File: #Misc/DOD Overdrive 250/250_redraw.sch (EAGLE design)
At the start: 21 parts, among them IC1 LM741, J1 IN, J2 OUT

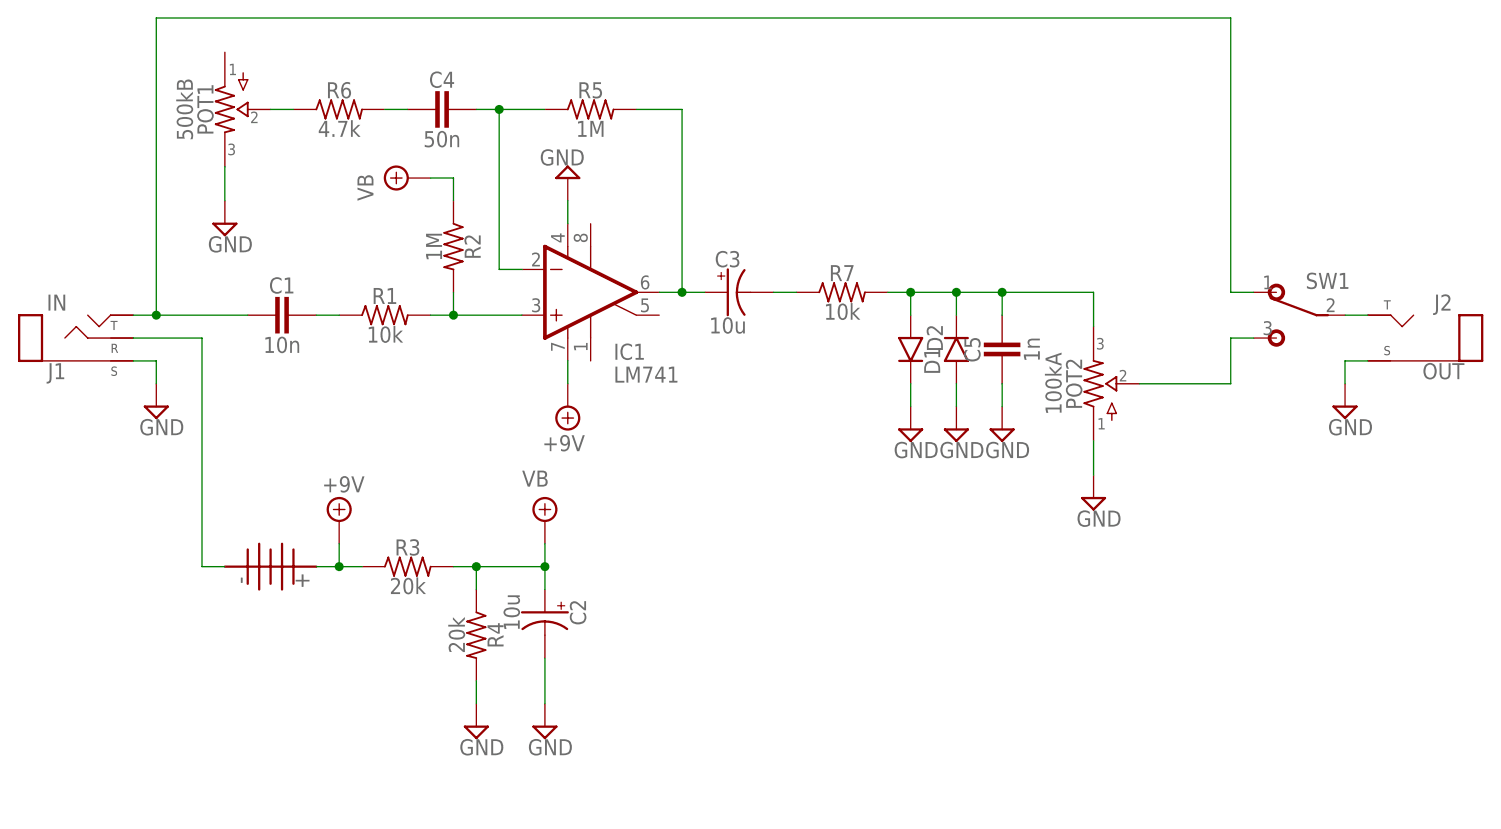
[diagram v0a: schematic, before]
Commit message: 20180125
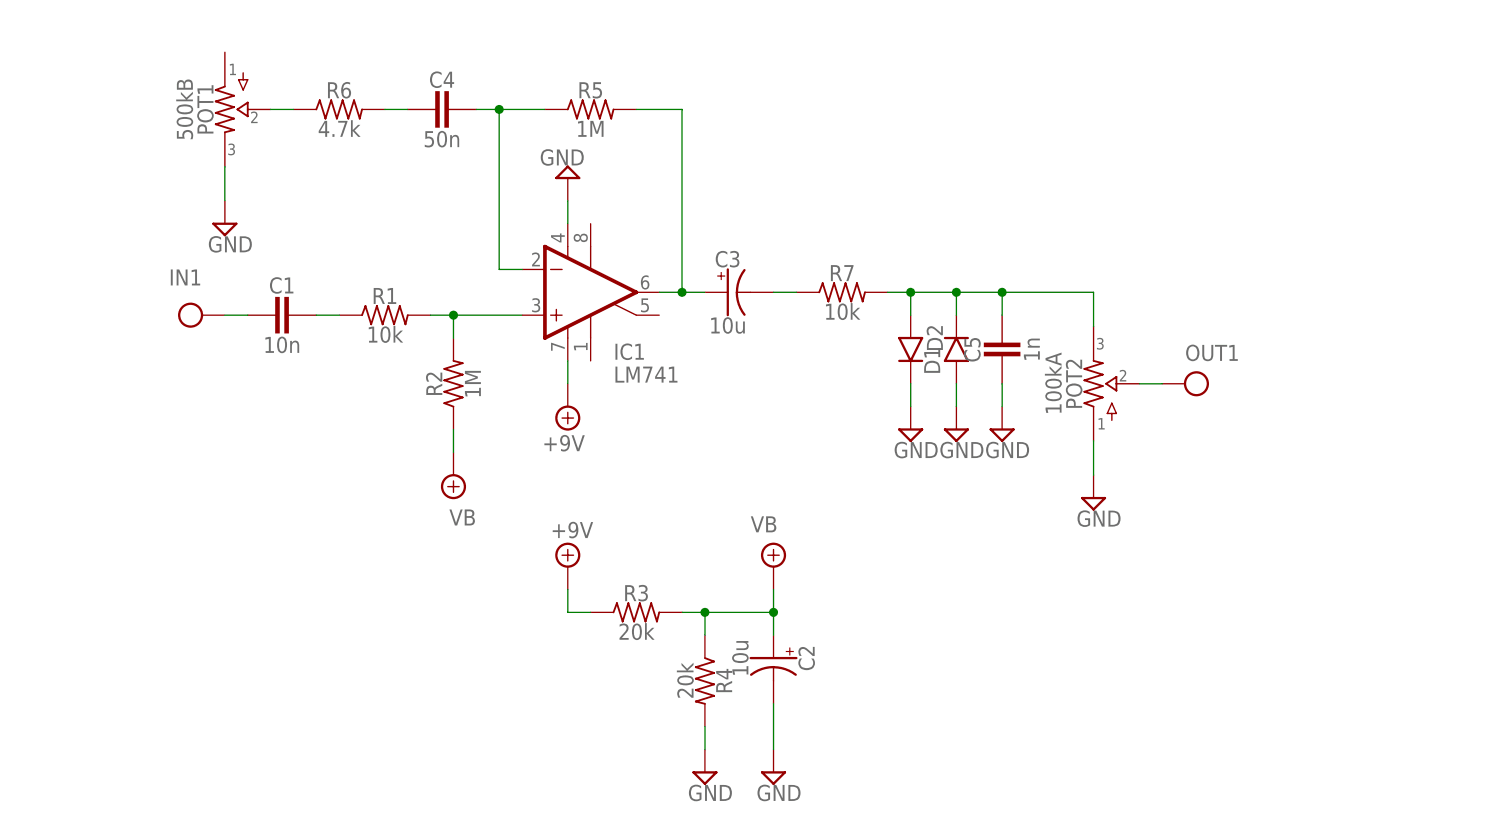
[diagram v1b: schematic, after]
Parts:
- removed 1: 9V, pedals-jacks:BATTERY
- removed J1: IN, pedals-jacks:STEREO
- removed J2: OUT, pedals-jacks:MONO_JACK
- removed SW1: (no value), pedals-switches:SPDT
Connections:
- removed net N$1: 1.P$2, J1.R
- removed net N$14: POT2.2, SW1.S
- removed net N$3: J1.T, SW1.O
- removed net N$6: J2.TIP, SW1.P
- new net IN: C1.2
- new net OUT: POT2.2
- net +9V: no longer 1.P$1
- net GND: no longer J1.S, J2.SLEEVE
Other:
- moved on the sheet: C2, R2, R3, R4
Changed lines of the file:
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@@
 <?xml version="1.0" encoding="utf-8"?>
 <!DOCTYPE eagle SYSTEM "eagle.dtd">
-<eagle version="8.2.0">
+<eagle version="8.5.1">
 <drawing>
 <settings>
 <setting alwaysvectorfont="no"/>
+<setting keepoldvectorfont="yes"/>
 <setting verticaltext="up"/>
 </settings>
-<grid distance="0.1" unitdist="inch" unit="inch" style="lines" multiple="1" display="yes" altdistance="0.01" altunitdist="inch" altunit="inch"/>
+<grid distance="0.1" unitdist="inch" unit="inch" style="lines" multiple="1" display="no" altdistance="0.01" altunitdist="inch" altunit="inch"/>
 <layers>
 <layer number="1" name="Top" color="4" fill="1" visible="no" active="no"/>
@@
 <layer number="59" name="tCarbon" color="7" fill="1" visible="no" active="no"/>
 <layer number="60" name="bCarbon" color="7" fill="1" visible="no" active="no"/>
+<layer number="88" name="SimResults" color="9" fill="1" visible="yes" active="yes"/>
+<layer number="89" name="SimProbes" color="9" fill="1" visible="yes" active="yes"/>
 <layer number="90" name="Modules" color="5" fill="1" visible="yes" active="yes"/>
 <layer number="91" name="Nets" color="2" fill="1" visible="yes" active="yes"/>
@@
 </classes>
 <parts>
-<part name="J1" library="pedals-jacks" deviceset="STEREO" device="" value="IN"/>
-<part name="GND1" library="gm-supply" deviceset="GND" device=""/>
-<part name="1" library="pedals-jacks" deviceset="BATTERY" device="" value="9V"/>
-<part name="J2" library="pedals-jacks" deviceset="MONO" device="_JACK" value="OUT"/>
 <part name="C1" library="pedals-capacitors-film" deviceset="CER/FILM" device="BOX.1" value="10n"/>
-<part name="SW1" library="pedals-switches" deviceset="SPDT" device=""/>
 <part name="R1" library="pedals-resistors" deviceset="R_" device=".3B" value="10k"/>
 <part name="R2" library="pedals-resistors" deviceset="R_" device=".3B" value="1M"/>
@@
 <part name="VB2" library="gm-supply" deviceset="VB" device=""/>
 <part name="V2" library="gm-supply" deviceset="+9V" device=""/>
-<part name="GND10" library="gm-supply" deviceset="GND" device=""/>
+<part name="IN1" library="pedals-supply" deviceset="IN" device=""/>
+<part name="OUT1" library="pedals-supply" deviceset="OUT" device=""/>
 </parts>
 <sheets>
@@
 </plain>
 <instances>
-<instance part="J1" gate="G$1" x="2.54" y="66.04" rot="MR180"/>
-<instance part="GND1" gate="GND" x="17.78" y="55.88"/>
-<instance part="1" gate="G$1" x="30.48" y="38.1" rot="R270"/>
-<instance part="J2" gate="G$1" x="157.48" y="63.5" rot="MR0"/>
 <instance part="C1" gate="G$1" x="31.75" y="66.04"/>
-<instance part="SW1" gate="1" x="144.78" y="68.58" rot="MR270"/>
 <instance part="R1" gate="G$1" x="43.18" y="66.04"/>
-<instance part="R2" gate="G$1" x="50.8" y="73.66" rot="R270"/>
-<instance part="R3" gate="G$1" x="45.72" y="38.1"/>
-<instance part="R4" gate="G$1" x="53.34" y="30.48" rot="R270"/>
-<instance part="C2" gate="1" x="60.96" y="33.02" rot="R270"/>
-<instance part="GND2" gate="GND" x="53.34" y="20.32"/>
+<instance part="R2" gate="G$1" x="50.8" y="58.42" rot="R90"/>
+<instance part="R3" gate="G$1" x="71.12" y="33.02"/>
+<instance part="R4" gate="G$1" x="78.74" y="25.4" rot="R270"/>
+<instance part="C2" gate="1" x="86.36" y="27.94" rot="R270"/>
+<instance part="GND2" gate="GND" x="78.74" y="15.24"/>
 <instance part="IC1" gate="A" x="66.04" y="68.58" rot="MR180"/>
 <instance part="GND3" gate="GND" x="63.5" y="81.28" rot="R180"/>
@@
 <instance part="GND7" gate="GND" x="111.76" y="53.34"/>
 <instance part="GND8" gate="GND" x="121.92" y="45.72"/>
-<instance part="GND9" gate="GND" x="60.96" y="20.32"/>
-<instance part="V1" gate="+9V" x="38.1" y="43.18"/>
-<instance part="VB1" gate="G$1" x="60.96" y="43.18"/>
-<instance part="VB2" gate="G$1" x="45.72" y="81.28" rot="R90"/>
+<instance part="GND9" gate="GND" x="86.36" y="15.24"/>
+<instance part="V1" gate="+9V" x="63.5" y="38.1"/>
+<instance part="VB1" gate="G$1" x="86.36" y="38.1"/>
+<instance part="VB2" gate="G$1" x="50.8" y="48.26" rot="R180"/>
 <instance part="V2" gate="+9V" x="63.5" y="55.88" rot="R180"/>
-<instance part="GND10" gate="GND" x="149.86" y="55.88"/>
+<instance part="IN1" gate="G$1" x="22.86" y="66.04"/>
+<instance part="OUT1" gate="G$1" x="132.08" y="58.42"/>
 </instances>
 <busses>
 </busses>
 <nets>
-<net name="N$1" class="0">
-<segment>
-<pinref part="J1" gate="G$1" pin="R"/>
-<wire x1="15.24" y1="63.5" x2="22.86" y2="63.5" width="0.1524" layer="91"/>
-<wire x1="22.86" y1="63.5" x2="22.86" y2="38.1" width="0.1524" layer="91"/>
-<pinref part="1" gate="G$1" pin="P$2"/>
-<wire x1="22.86" y1="38.1" x2="25.4" y2="38.1" width="0.1524" layer="91"/>
-</segment>
-</net>
-<net name="N$3" class="0">
-<segment>
-<pinref part="J1" gate="G$1" pin="T"/>
-<wire x1="15.24" y1="66.04" x2="17.78" y2="66.04" width="0.1524" layer="91"/>
-<pinref part="SW1" gate="1" pin="O"/>
-<wire x1="17.78" y1="66.04" x2="27.94" y2="66.04" width="0.1524" layer="91"/>
-<wire x1="139.7" y1="68.58" x2="137.16" y2="68.58" width="0.1524" layer="91"/>
-<wire x1="137.16" y1="68.58" x2="137.16" y2="99.06" width="0.1524" layer="91"/>
-<wire x1="137.16" y1="99.06" x2="17.78" y2="99.06" width="0.1524" layer="91"/>
-<wire x1="17.78" y1="99.06" x2="17.78" y2="66.04" width="0.1524" layer="91"/>
-<junction x="17.78" y="66.04"/>
-</segment>
-</net>
 <net name="GND" class="0">
-<segment>
-<pinref part="J1" gate="G$1" pin="S"/>
-<pinref part="GND1" gate="GND" pin="GND"/>
-<wire x1="15.24" y1="60.96" x2="17.78" y2="60.96" width="0.1524" layer="91"/>
-<wire x1="17.78" y1="60.96" x2="17.78" y2="58.42" width="0.1524" layer="91"/>
-</segment>
 <segment>
 <pinref part="GND4" gate="GND" pin="GND"/>
@@
 </segment>
 <segment>
-<pinref part="GND10" gate="GND" pin="GND"/>
-<wire x1="149.86" y1="58.42" x2="149.86" y2="60.96" width="0.1524" layer="91"/>
-<pinref part="J2" gate="G$1" pin="SLEEVE"/>
-<wire x1="149.86" y1="60.96" x2="152.4" y2="60.96" width="0.1524" layer="91"/>
-</segment>
-<segment>
 <pinref part="GND2" gate="GND" pin="GND"/>
 <pinref part="R4" gate="G$1" pin="2"/>
-<wire x1="53.34" y1="22.86" x2="53.34" y2="25.4" width="0.1524" layer="91"/>
+<wire x1="78.74" y1="17.78" x2="78.74" y2="20.32" width="0.1524" layer="91"/>
 </segment>
 <segment>
 <pinref part="GND9" gate="GND" pin="GND"/>
 <pinref part="C2" gate="1" pin="-"/>
-<wire x1="60.96" y1="22.86" x2="60.96" y2="27.94" width="0.1524" layer="91"/>
+<wire x1="86.36" y1="17.78" x2="86.36" y2="22.86" width="0.1524" layer="91"/>
 </segment>
 </net>
@@
 <pinref part="R2" gate="G$1" pin="2"/>
 <wire x1="48.26" y1="66.04" x2="50.8" y2="66.04" width="0.1524" layer="91"/>
-<wire x1="50.8" y1="66.04" x2="50.8" y2="68.58" width="0.1524" layer="91"/>
+<wire x1="50.8" y1="66.04" x2="50.8" y2="63.5" width="0.1524" layer="91"/>
 <junction x="50.8" y="66.04"/>
 <pinref part="IC1" gate="A" pin="+IN"/>
@@
 </segment>
 </net>
-<net name="N$14" class="0">
-<segment>
-<pinref part="POT2" gate="G$1" pin="2"/>
-<wire x1="127" y1="58.42" x2="137.16" y2="58.42" width="0.1524" layer="91"/>
-<wire x1="137.16" y1="58.42" x2="137.16" y2="63.5" width="0.1524" layer="91"/>
-<pinref part="SW1" gate="1" pin="S"/>
-<wire x1="137.16" y1="63.5" x2="139.7" y2="63.5" width="0.1524" layer="91"/>
-</segment>
-</net>
 <net name="+9V" class="0">
 <segment>
-<pinref part="1" gate="G$1" pin="P$1"/>
 <pinref part="R3" gate="G$1" pin="1"/>
-<wire x1="35.56" y1="38.1" x2="38.1" y2="38.1" width="0.1524" layer="91"/>
 <pinref part="V1" gate="+9V" pin="+9V"/>
-<wire x1="38.1" y1="38.1" x2="40.64" y2="38.1" width="0.1524" layer="91"/>
-<wire x1="38.1" y1="40.64" x2="38.1" y2="38.1" width="0.1524" layer="91"/>
-<junction x="38.1" y="38.1"/>
+<wire x1="63.5" y1="33.02" x2="66.04" y2="33.02" width="0.1524" layer="91"/>
+<wire x1="63.5" y1="35.56" x2="63.5" y2="33.02" width="0.1524" layer="91"/>
 </segment>
 <segment>
@@
 <segment>
 <pinref part="R3" gate="G$1" pin="2"/>
-<wire x1="60.96" y1="38.1" x2="53.34" y2="38.1" width="0.1524" layer="91"/>
+<wire x1="86.36" y1="33.02" x2="78.74" y2="33.02" width="0.1524" layer="91"/>
 <pinref part="VB1" gate="G$1" pin="VB"/>
-<wire x1="53.34" y1="38.1" x2="50.8" y2="38.1" width="0.1524" layer="91"/>
-<wire x1="60.96" y1="40.64" x2="60.96" y2="38.1" width="0.1524" layer="91"/>
+<wire x1="78.74" y1="33.02" x2="76.2" y2="33.02" width="0.1524" layer="91"/>
+<wire x1="86.36" y1="35.56" x2="86.36" y2="33.02" width="0.1524" layer="91"/>
 <pinref part="C2" gate="1" pin="+"/>
-<wire x1="60.96" y1="35.56" x2="60.96" y2="38.1" width="0.1524" layer="91"/>
+<wire x1="86.36" y1="30.48" x2="86.36" y2="33.02" width="0.1524" layer="91"/>
 <pinref part="R4" gate="G$1" pin="1"/>
-<wire x1="53.34" y1="35.56" x2="53.34" y2="38.1" width="0.1524" layer="91"/>
-<junction x="53.34" y="38.1"/>
-<junction x="60.96" y="38.1"/>
+<wire x1="78.74" y1="30.48" x2="78.74" y2="33.02" width="0.1524" layer="91"/>
+<junction x="78.74" y="33.02"/>
+<junction x="86.36" y="33.02"/>
 </segment>
 <segment>
 <pinref part="VB2" gate="G$1" pin="VB"/>
 <pinref part="R2" gate="G$1" pin="1"/>
-<wire x1="48.26" y1="81.28" x2="50.8" y2="81.28" width="0.1524" layer="91"/>
-<wire x1="50.8" y1="81.28" x2="50.8" y2="78.74" width="0.1524" layer="91"/>
-</segment>
-</net>
-<net name="N$6" class="0">
-<segment>
-<pinref part="SW1" gate="1" pin="P"/>
-<pinref part="J2" gate="G$1" pin="TIP"/>
-<wire x1="149.86" y1="66.04" x2="152.4" y2="66.04" width="0.1524" layer="91"/>
-</segment>
-</net>
+<wire x1="50.8" y1="50.8" x2="50.8" y2="53.34" width="0.1524" layer="91"/>
+</segment>
+</net>
+<net name="IN" class="0">
+<segment>
+<pinref part="IN1" gate="G$1" pin="IN"/>
+<pinref part="C1" gate="G$1" pin="2"/>
+<wire x1="25.4" y1="66.04" x2="27.94" y2="66.04" width="0.1524" layer="91"/>
+</segment>
+</net>
+<net name="OUT" class="0">
+<segment>
+<pinref part="POT2" gate="G$1" pin="2"/>
+<pinref part="OUT1" gate="G$1" pin="OUT"/>
+<wire x1="127" y1="58.42" x2="129.54" y2="58.42" width="0.1524" layer="91"/>
+</segment>
+</net>
